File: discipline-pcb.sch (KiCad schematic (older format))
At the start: 171 parts, among them J1 AVR-ISP-6, SW0 KEYSW, SW1 KEYSW, SW10 KEYSW, SW11 KEYSW, SW12 KEYSW, SW13 KEYSW, SW14 KEYSW, SW15 KEYSW, SW16 KEYSW, SW17 KEYSW, SW18 KEYSW, SW19 KEYSW, SW2 KEYSW, SW20 KEYSW, SW21 KEYSW, SW22 KEYSW, SW23 KEYSW, SW24 KEYSW, SW25 KEYSW, SW26 KEYSW, SW27 KEYSW, SW28 KEYSW, SW29 KEYSW, SW3 KEYSW, SW30 KEYSW, SW31 KEYSW, SW32 KEYSW, SW33 KEYSW, SW34 KEYSW, SW35 KEYSW, SW36 KEYSW, SW37 KEYSW, SW38 KEYSW, SW39 KEYSW, SW4 KEYSW, SW40 KEYSW, SW41 KEYSW, SW42 KEYSW, SW43 KEYSW, SW44 KEYSW, SW45 KEYSW, SW46 KEYSW, SW47 KEYSW, SW48 KEYSW, SW49 KEYSW, SW5 KEYSW, SW50 KEYSW, SW51 KEYSW, SW52 KEYSW, SW53 KEYSW, SW54 KEYSW, SW55 KEYSW, SW56 KEYSW, SW57 KEYSW, SW58 KEYSW, SW59 KEYSW, SW6 KEYSW, SW60 KEYSW, SW61 KEYSW, SW62 KEYSW, SW63 KEYSW, SW64 KEYSW, SW65 KEYSW, SW66 KEYSW, SW67 KEYSW, SW68 KEYSW, SW69 KEYSW, SW7 KEYSW, SW70 KEYSW, SW71 KEYSW, SW72 KEYSW, SW73 KEYSW, SW74 KEYSW, SW75 KEYSW, SW76 KEYSW, SW77 KEYSW, SW78 KEYSW, SW8 KEYSW, SW9 KEYSW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

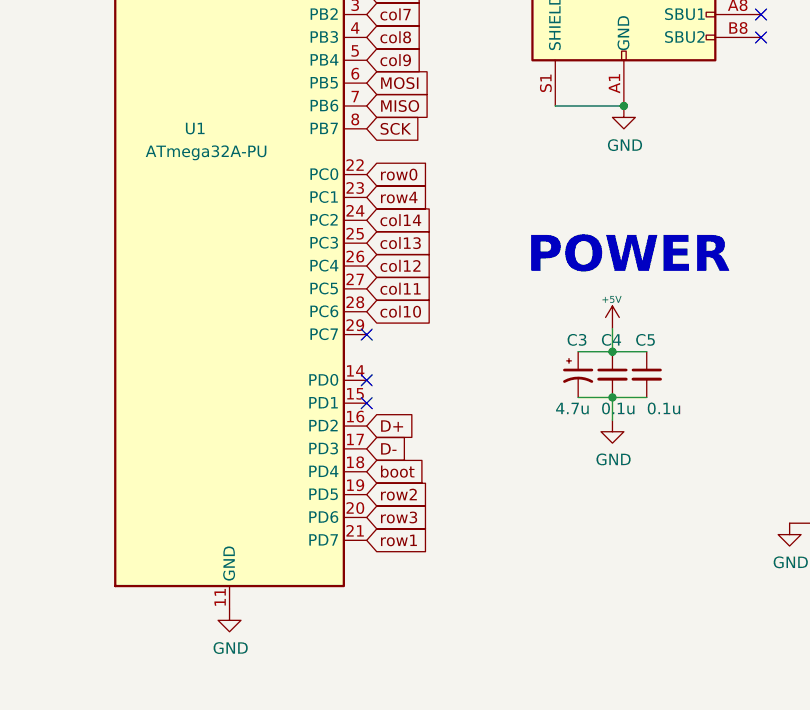
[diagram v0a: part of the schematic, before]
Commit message: Last cleanup of placements.
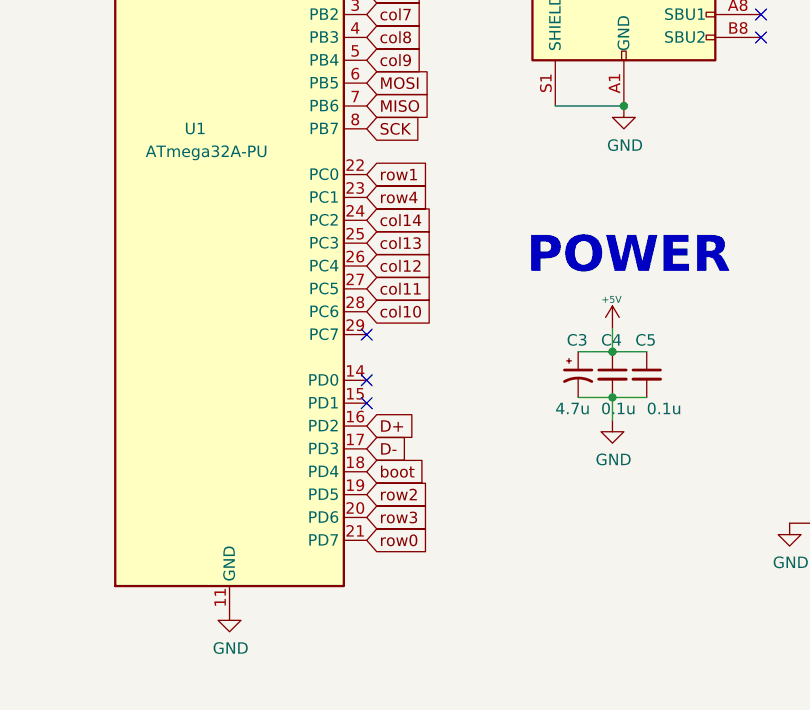
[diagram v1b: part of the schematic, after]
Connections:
- net row0: now also U1.21 (PD7); no longer U1.22 (PC0)
- net row1: now also U1.22 (PC0); no longer U1.21 (PD7)
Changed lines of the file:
@@
 Text GLabel 4575 10300 2    50   Input ~ 0
 row3
-Text GLabel 4575 8800 2    50   Input ~ 0
+Text GLabel 4575 10400 2    50   Input ~ 0
 row0
 Text GLabel 4575 7000 2    50   Input ~ 0
@@
 Text Label 3900 3100 0    50   ~ 0
 col0
-Text GLabel 4575 10400 2    50   Input ~ 0
+Text GLabel 4575 8800 2    50   Input ~ 0
 row1
 Text GLabel 4575 10200 2    50   Input ~ 0

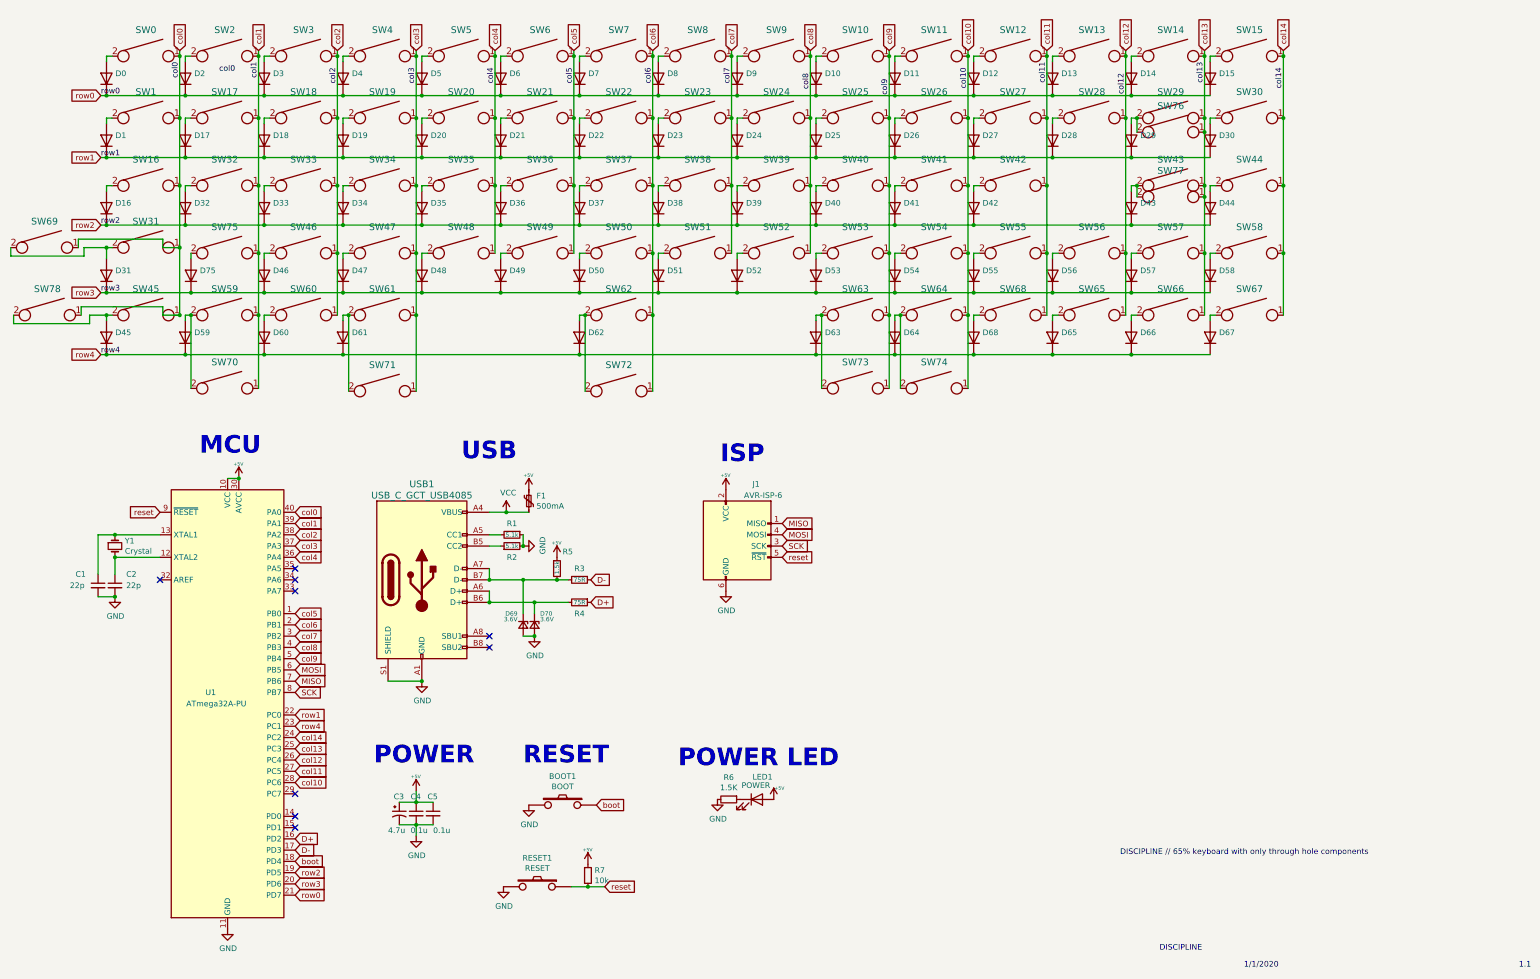
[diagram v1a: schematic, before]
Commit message: Wrapping Up
Finished up all major tasks.
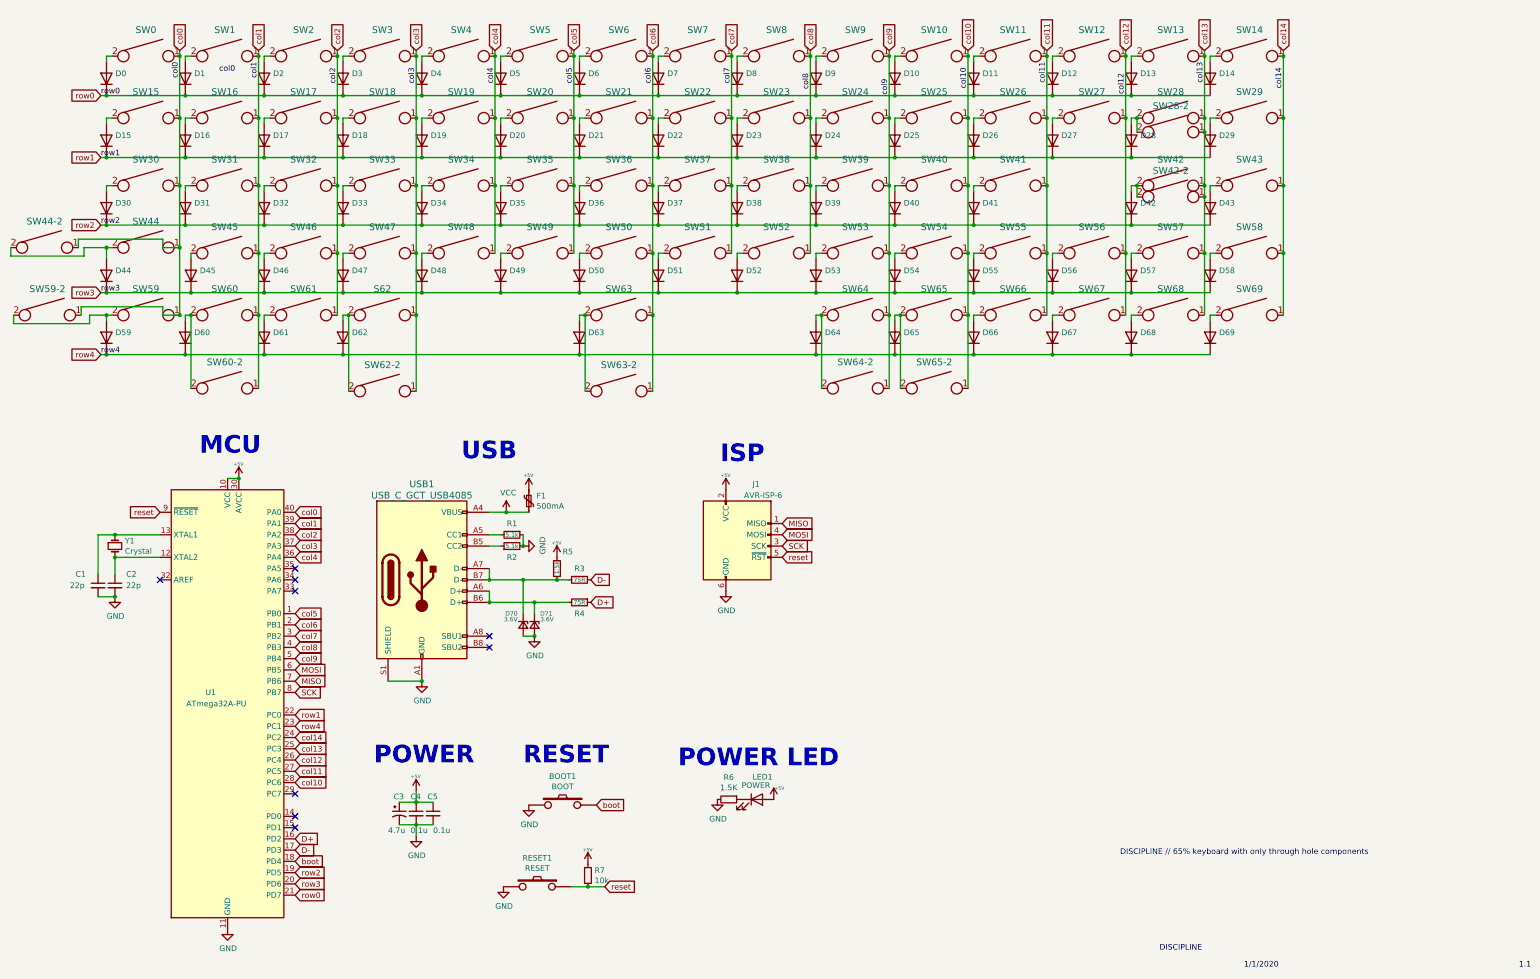
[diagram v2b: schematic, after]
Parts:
- renumbered D2 to D1, D11 to D10, D12 to D11, D13 to D12, D14 to D13, D15 to D14, D1 to D15, D17 to D16, D18 to D17, D19 to D18, D20 to D19, D3 to D2, D21 to D20, D22 to D21, D23 to D22, D24 to D23, D25 to D24, D26 to D25, D27 to D26, D28 to D27, D29 to D28, D30 to D29, D4 to D3, D16 to D30, D32 to D31, D33 to D32, D34 to D33, D35 to D34, D36 to D35, D37 to D36, D38 to D37, D39 to D38, D40 to D39, D5 to D4, D41 to D40, D42 to D41, D43 to D42, D44 to D43, D31 to D44, D75 to D45, D6 to D5, D45 to D59, D7 to D6, D59 to D60, D60 to D61, D61 to D62, D62 to D63, D63 to D64, D64 to D65, D68 to D66, D65 to D67, D66 to D68, D67 to D69, D8 to D7, D69 to D70, D70 to D71, D9 to D8, D10 to D9, SW61 to S62, SW2 to SW1, SW11 to SW10, SW12 to SW11, SW13 to SW12, SW14 to SW13, SW15 to SW14, SW1 to SW15, SW17 to SW16, SW18 to SW17, SW19 to SW18, SW20 to SW19, SW3 to SW2, SW21 to SW20, SW22 to SW21, SW23 to SW22, SW24 to SW23, SW25 to SW24, SW26 to SW25, SW27 to SW26, SW28 to SW27, SW29 to SW28, SW76 to SW28-2, SW30 to SW29, SW4 to SW3, SW16 to SW30, SW32 to SW31, SW33 to SW32, SW34 to SW33, SW35 to SW34, SW36 to SW35, SW37 to SW36, SW38 to SW37, SW39 to SW38, SW40 to SW39, SW5 to SW4, SW41 to SW40, SW42 to SW41, SW43 to SW42, SW77 to SW42-2, SW44 to SW43, SW31 to SW44, SW69 to SW44-2, SW75 to SW45, SW6 to SW5, SW45 to SW59, SW78 to SW59-2, SW7 to SW6, SW59 to SW60, SW70 to SW60-2, SW60 to SW61, SW71 to SW62-2, SW62 to SW63, SW72 to SW63-2, SW63 to SW64, SW73 to SW64-2, SW64 to SW65, SW74 to SW65-2, SW68 to SW66, SW65 to SW67, SW66 to SW68, SW67 to SW69, SW8 to SW7, SW9 to SW8, SW10 to SW9
